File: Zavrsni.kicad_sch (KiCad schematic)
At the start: 42 parts, among them SW1 SW_Push, SW2 SW_Push

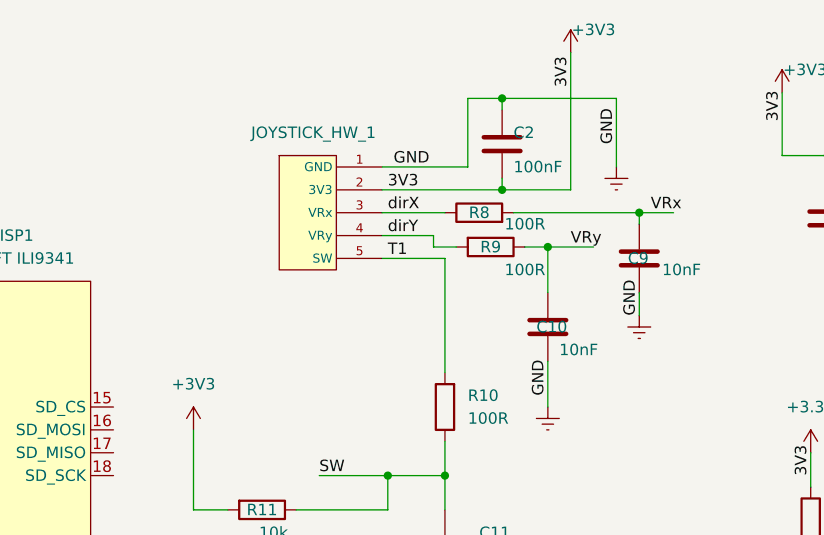
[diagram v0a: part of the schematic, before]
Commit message: Finnal version of PCB and schema
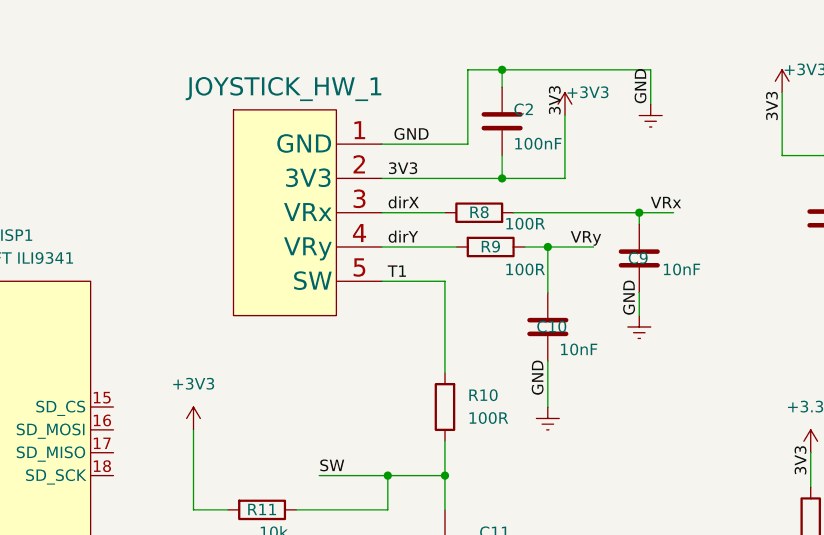
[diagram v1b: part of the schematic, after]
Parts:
- removed JOYSTICK_HW_1: ~, JOYSTICK:JOYSTICK, symbol joystick_symbol1:JOYSTICK-HW-504
- added JOYSTICK_HW_1: ~, JOYSTICK:JOYSTICK, symbol JOYSTICK_symbol:joystick_HW_504
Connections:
- net +3.3V: now also JOYSTICK_HW_1.2 (3V3)
- net Earth: now also JOYSTICK_HW_1.1 (GND)
- net T1: now also JOYSTICK_HW_1.5 (SW)
- net dirX: now also JOYSTICK_HW_1.3 (VRx)
- net dirY: now also JOYSTICK_HW_1.4 (VRy)
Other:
- moved on the sheet: C2
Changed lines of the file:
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@@
   (junction (at 139.065 151.13) (diameter 0) (color 0 0 0 0)
   )
-  (junction (at 153.67 29.21) (diameter 0) (color 0 0 0 0)
+  (junction (at 153.67 26.035) (diameter 0) (color 0 0 0 0)
   )
   (junction (at 204.47 35.56) (diameter 0) (color 0 0 0 0)
@@
   (junction (at 197.485 35.56) (diameter 0) (color 0 0 0 0)
   )
+  (junction (at 153.67 38.1) (diameter 0) (color 0 0 0 0)
+  )
   (junction (at 131.445 134.62) (diameter 0) (color 0 0 0 0)
   )
@@
   (junction (at 140.97 71.12) (diameter 0) (color 0 0 0 0)
   )
-  (junction (at 153.67 39.37) (diameter 0) (color 0 0 0 0)
-  )
   (junction (at 62.23 45.72) (diameter 0) (color 0 0 0 0)
   )
@@
     (stroke (width 0) (type default))
   )
-  (wire (pts (xy 153.67 29.21) (xy 153.67 30.48))
+  (wire (pts (xy 153.67 26.035) (xy 153.67 27.94))
     (stroke (width 0) (type default))
   )
@@
     (stroke (width 0) (type default))
   )
-  (wire (pts (xy 149.86 29.21) (xy 153.67 29.21))
+  (wire (pts (xy 149.86 26.035) (xy 153.67 26.035))
     (stroke (width 0) (type default))
   )
@@
     (stroke (width 0) (type default))
   )
-  (wire (pts (xy 153.67 39.37) (xy 161.29 39.37))
+  (wire (pts (xy 153.67 38.1) (xy 160.655 38.1))
     (stroke (width 0) (type default))
   )
@@
     (stroke (width 0) (type default))
   )
-  (wire (pts (xy 166.37 29.21) (xy 166.37 36.83))
+  (wire (pts (xy 170.18 26.035) (xy 170.18 29.845))
     (stroke (width 0) (type default))
   )
@@
     (stroke (width 0) (type default))
   )
-  (wire (pts (xy 140.335 39.37) (xy 153.67 39.37))
+  (wire (pts (xy 140.335 38.1) (xy 153.67 38.1))
     (stroke (width 0) (type default))
   )
@@
     (stroke (width 0) (type default))
   )
-  (wire (pts (xy 153.67 38.1) (xy 153.67 39.37))
+  (wire (pts (xy 153.67 35.56) (xy 153.67 38.1))
     (stroke (width 0) (type default))
   )
@@
     (stroke (width 0) (type default))
   )
-  (wire (pts (xy 149.86 29.21) (xy 149.86 36.83))
+  (wire (pts (xy 149.86 26.035) (xy 149.86 34.29))
     (stroke (width 0) (type default))
   )
@@
     (stroke (width 0) (type default))
   )
-  (wire (pts (xy 161.29 24.13) (xy 161.29 39.37))
+  (wire (pts (xy 160.655 31.115) (xy 160.655 38.1))
     (stroke (width 0) (type default))
   )
@@
     (stroke (width 0) (type default))
   )
-  (wire (pts (xy 147.32 46.99) (xy 147.32 59.69))
+  (wire (pts (xy 147.32 49.53) (xy 147.32 59.69))
     (stroke (width 0) (type default))
   )
@@
     (stroke (width 0) (type default))
   )
-  (wire (pts (xy 153.67 29.21) (xy 166.37 29.21))
+  (wire (pts (xy 153.67 26.035) (xy 170.18 26.035))
     (stroke (width 0) (type default))
   )
@@
     (stroke (width 0) (type default))
   )
-  (wire (pts (xy 140.335 44.45) (xy 146.05 44.45))
+  (wire (pts (xy 140.335 45.72) (xy 148.59 45.72))
     (stroke (width 0) (type default))
   )
@@
     (stroke (width 0) (type default))
   )
-  (wire (pts (xy 140.335 46.99) (xy 147.32 46.99))
+  (wire (pts (xy 140.335 49.53) (xy 147.32 49.53))
     (stroke (width 0) (type default))
   )
@@
     (stroke (width 0) (type default))
   )
-  (wire (pts (xy 146.05 45.72) (xy 148.59 45.72))
-    (stroke (width 0) (type default))
-  )
   (wire (pts (xy 123.825 134.62) (xy 123.825 170.18))
     (stroke (width 0) (type default))
@@
     (stroke (width 0) (type default))
   )
-  (wire (pts (xy 146.05 44.45) (xy 146.05 45.72))
-    (stroke (width 0) (type default))
-  )
-  (wire (pts (xy 140.335 36.83) (xy 149.86 36.83))
+  (wire (pts (xy 140.335 34.29) (xy 149.86 34.29))
     (stroke (width 0) (type default))
   )
@@
     (effects (font (size 1.27 1.27)) (justify left bottom))
   )
-  (label "3V3" (at 140.97 39.37 0) (fields_autoplaced)
+  (label "3V3" (at 140.97 38.1 0) (fields_autoplaced)
     (effects (font (size 1.27 1.27)) (justify left bottom))
   )
@@
     (effects (font (size 1.27 1.27)) (justify left bottom))
   )
-  (label "3V3" (at 161.29 27.94 90) (fields_autoplaced)
+  (label "3V3" (at 160.655 31.115 90) (fields_autoplaced)
     (effects (font (size 1.27 1.27)) (justify left bottom))
   )
@@
     (effects (font (size 1.27 1.27)) (justify left bottom))
   )
-  (label "dirY" (at 140.97 44.45 0) (fields_autoplaced)
+  (label "dirY" (at 140.97 45.72 0) (fields_autoplaced)
     (effects (font (size 1.27 1.27)) (justify left bottom))
   )
@@
     (effects (font (size 1.27 1.27)) (justify left bottom))
   )
-  (label "GND" (at 141.605 36.83 0) (fields_autoplaced)
+  (label "GND" (at 141.605 34.29 0) (fields_autoplaced)
     (effects (font (size 1.27 1.27)) (justify left bottom))
   )
@@
     (effects (font (size 1.27 1.27)) (justify left bottom))
   )
-  (label "GND" (at 166.37 34.29 90) (fields_autoplaced)
+  (label "GND" (at 170.18 29.845 90) (fields_autoplaced)
     (effects (font (size 1.27 1.27)) (justify left bottom))
   )
@@
     (effects (font (size 1.27 1.27)) (justify left bottom))
   )
-  (label "T1" (at 140.97 46.99 0) (fields_autoplaced)
+  (label "T1" (at 140.97 49.53 0) (fields_autoplaced)
     (effects (font (size 1.27 1.27)) (justify left bottom))
   )
@@
         (path "/0b0be7ad-a3a6-4dc5-99d9-af21078bf390"
           (reference "R1") (unit 1)
-        )
-      )
-    )
-  )
-  (symbol (lib_id "joystick_symbol1:JOYSTICK-HW-504") (at 132.715 40.64 0) (unit 1)
-    (in_bom yes) (on_board yes) (dnp no) (fields_autoplaced)
-    (property "Reference" "JOYSTICK_HW_1" (at 132.715 33.02 0)
-      (effects (font (size 1.27 1.27)))
-    )
-    (property "Value" "~" (at 132.715 40.64 0)
-      (effects (font (size 1.27 1.27)))
-    )
-    (property "Footprint" "JOYSTICK:JOYSTICK" (at 132.715 40.64 0)
-      (effects (font (size 1.27 1.27)) hide)
-    )
-    (property "Datasheet" "" (at 132.715 40.64 0)
-      (effects (font (size 1.27 1.27)) hide)
-    )
-    (pin "1")
-    (pin "2")
-    (pin "3")
-    (pin "4")
-    (pin "5")
-    (instances
-      (project "Zavrsni"
-        (path "/0b0be7ad-a3a6-4dc5-99d9-af21078bf390"
-          (reference "JOYSTICK_HW_1") (unit 1)
         )
       )
@@
     )
   )
-  (symbol (lib_id "power:+3V3") (at 161.29 24.13 0) (unit 1)
-    (in_bom yes) (on_board yes) (dnp no)
-    (property "Reference" "#PWR03" (at 161.29 27.94 0)
-      (effects (font (size 1.27 1.27)) hide)
-    )
-    (property "Value" "+3V3" (at 163.83 21.59 0)
-      (effects (font (size 1.27 1.27)))
-    )
-    (property "Footprint" "" (at 161.29 24.13 0)
-      (effects (font (size 1.27 1.27)) hide)
-    )
-    (property "Datasheet" "" (at 161.29 24.13 0)
+  (symbol (lib_id "power:+3V3") (at 160.655 31.115 0) (unit 1)
+    (in_bom yes) (on_board yes) (dnp no)
+    (property "Reference" "#PWR03" (at 160.655 34.925 0)
+      (effects (font (size 1.27 1.27)) hide)
+    )
+    (property "Value" "+3V3" (at 163.195 28.575 0)
+      (effects (font (size 1.27 1.27)))
+    )
+    (property "Footprint" "" (at 160.655 31.115 0)
+      (effects (font (size 1.27 1.27)) hide)
+    )
+    (property "Datasheet" "" (at 160.655 31.115 0)
       (effects (font (size 1.27 1.27)) hide)
     )
@@
     )
   )
-  (symbol (lib_id "power:Earth") (at 166.37 36.83 0) (unit 1)
-    (in_bom yes) (on_board yes) (dnp no) (fields_autoplaced)
-    (property "Reference" "#PWR08" (at 166.37 43.18 0)
-      (effects (font (size 1.27 1.27)) hide)
-    )
-    (property "Value" "Earth" (at 166.37 40.64 0)
-      (effects (font (size 1.27 1.27)) hide)
-    )
-    (property "Footprint" "" (at 166.37 36.83 0)
-      (effects (font (size 1.27 1.27)) hide)
-    )
-    (property "Datasheet" "~" (at 166.37 36.83 0)
+  (symbol (lib_id "power:Earth") (at 170.18 29.845 0) (unit 1)
+    (in_bom yes) (on_board yes) (dnp no) (fields_autoplaced)
+    (property "Reference" "#PWR08" (at 170.18 36.195 0)
+      (effects (font (size 1.27 1.27)) hide)
+    )
+    (property "Value" "Earth" (at 170.18 33.655 0)
+      (effects (font (size 1.27 1.27)) hide)
+    )
+    (property "Footprint" "" (at 170.18 29.845 0)
+      (effects (font (size 1.27 1.27)) hide)
+    )
+    (property "Datasheet" "~" (at 170.18 29.845 0)
       (effects (font (size 1.27 1.27)) hide)
     )
@@
     )
   )
-  (symbol (lib_id "Device:C") (at 153.67 34.29 0) (unit 1)
-    (in_bom yes) (on_board yes) (dnp no)
-    (property "Reference" "C2" (at 154.94 33.02 0)
-      (effects (font (size 1.27 1.27)) (justify left))
-    )
-    (property "Value" "100nF" (at 154.94 36.83 0)
-      (effects (font (size 1.27 1.27)) (justify left))
-    )
-    (property "Footprint" "Capacitor_SMD:C_0603_1608Metric" (at 154.6352 38.1 0)
-      (effects (font (size 1.27 1.27)) hide)
-    )
-    (property "Datasheet" "~" (at 153.67 34.29 0)
+  (symbol (lib_id "Device:C") (at 153.67 31.75 0) (unit 1)
+    (in_bom yes) (on_board yes) (dnp no)
+    (property "Reference" "C2" (at 154.94 30.48 0)
+      (effects (font (size 1.27 1.27)) (justify left))
+    )
+    (property "Value" "100nF" (at 154.94 34.29 0)
+      (effects (font (size 1.27 1.27)) (justify left))
+    )
+    (property "Footprint" "Capacitor_SMD:C_0603_1608Metric" (at 154.6352 35.56 0)
+      (effects (font (size 1.27 1.27)) hide)
+    )
+    (property "Datasheet" "~" (at 153.67 31.75 0)
       (effects (font (size 1.27 1.27)) hide)
     )
@@
         )
       )
+    )
+  )
+  (symbol (lib_id "JOYSTICK_symbol:joystick_HW_504") (at 130.175 41.91 0) (unit 1)
+    (in_bom yes) (on_board yes) (dnp no) (fields_autoplaced)
+    (property "Reference" "JOYSTICK_HW_1" (at 129.58 27.94 0)
+      (effects (font (size 2 2)))
+    )
+    (property "Value" "~" (at 132.715 81.28 0)
+      (effects (font (size 1.27 1.27)))
+    )
+    (property "Footprint" "JOYSTICK:JOYSTICK" (at 132.715 81.28 0)
+      (effects (font (size 1.27 1.27)) hide)
+    )
+    (property "Datasheet" "" (at 132.715 81.28 0)
+      (effects (font (size 1.27 1.27)) hide)
+    )
+    (pin "1")
+    (pin "2")
+    (pin "3")
+    (pin "4")
+    (pin "5")
+    (instances
+      (project "Zavrsni"
+        (path "/0b0be7ad-a3a6-4dc5-99d9-af21078bf390"
+          (reference "JOYSTICK_HW_1") (unit 1)
+        )
+      )
